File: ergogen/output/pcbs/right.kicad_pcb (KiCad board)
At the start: 2 copper layers, 140.9 x 96.1 mm, 88 parts

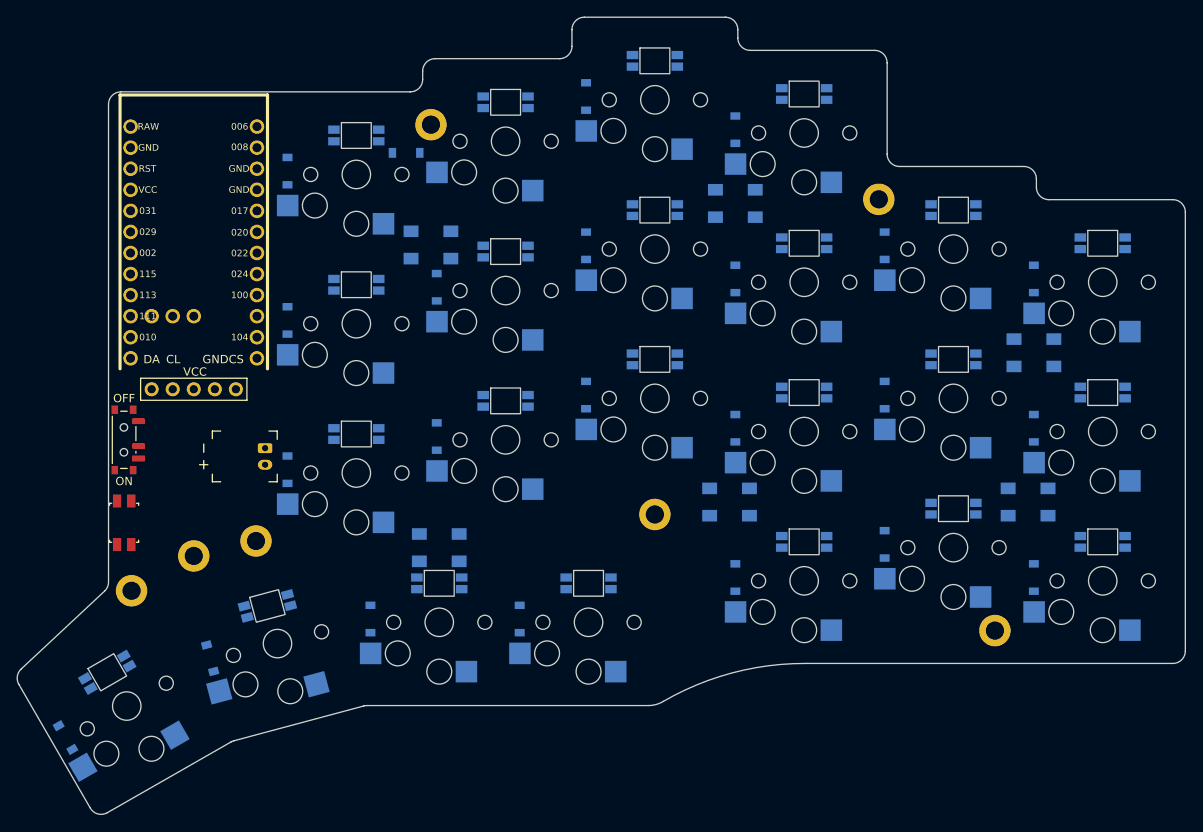
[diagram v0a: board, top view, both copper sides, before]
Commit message: wip: v2
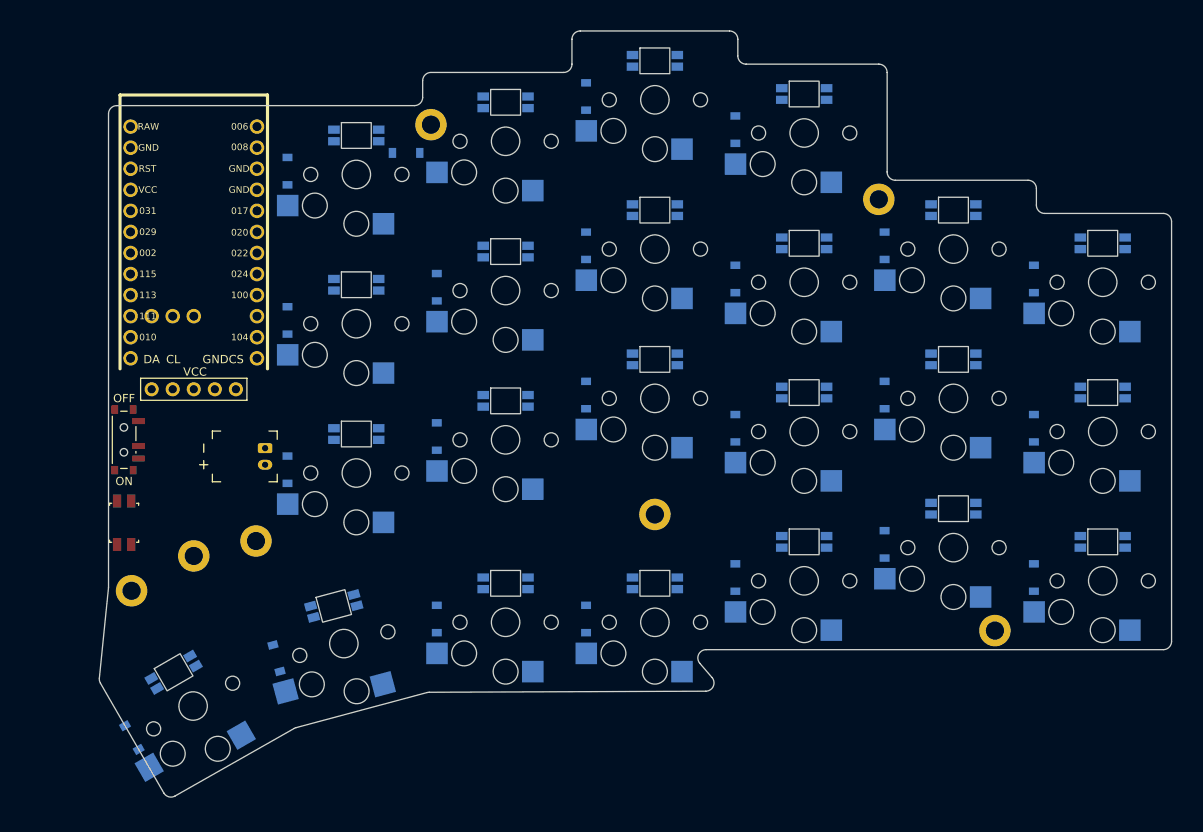
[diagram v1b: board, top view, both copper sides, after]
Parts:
- removed LED24, LED25, LED26, LED27, LED28, LED29: VAL**, WS2812B
- moved G 21.4 mm to (156.2, 173.4)
- moved LED23 8.00 mm to (138.0, 183.0)
- moved S23 8.00 mm to (140.3, 187.1)
- moved S22 8.00 mm to (158.5, 179.6)
- moved D21 8.00 mm to (150.4, 181.3)
- moved D19 8.00 mm to (187.7, 176.6)
- moved D20 8.00 mm to (169.7, 176.6)
- moved LED20 8.00 mm to (196.0, 172.3)
- moved LED21 8.00 mm to (178.0, 172.3)
- moved S20 8.00 mm to (196.0, 177.0)
- moved S21 8.00 mm to (178.0, 177.0)
- moved LED22 8.00 mm to (157.3, 175.0)
- moved D22 8.00 mm to (132.9, 190.9)
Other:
- board size 140.9 x 96.1 mm -> 129.3 x 92.4 mm
- net class Default added: clearance 0.2, trace_width 0.25, via_dia 0.8, via_drill 0.4
